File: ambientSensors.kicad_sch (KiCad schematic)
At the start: 14 parts, among them J2 BM04B-SRSS-TB, U1 LTR-329ALS-01, U3 TPS22914BYFPR, U7 BME688

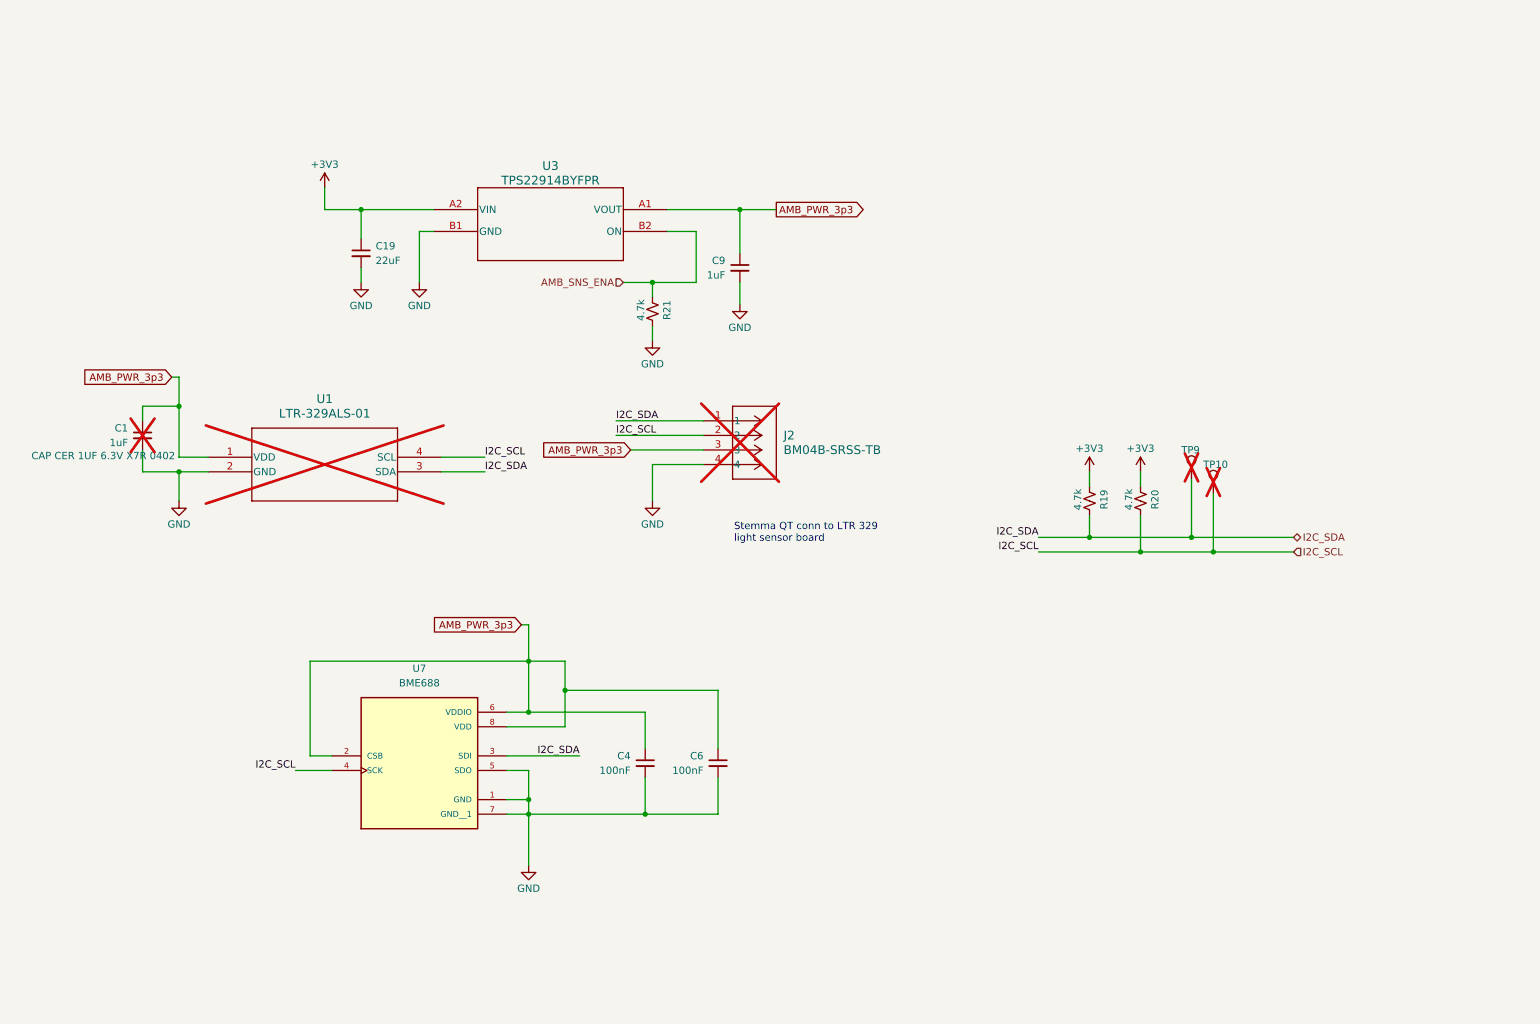
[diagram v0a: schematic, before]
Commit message: mutli soil sensor update
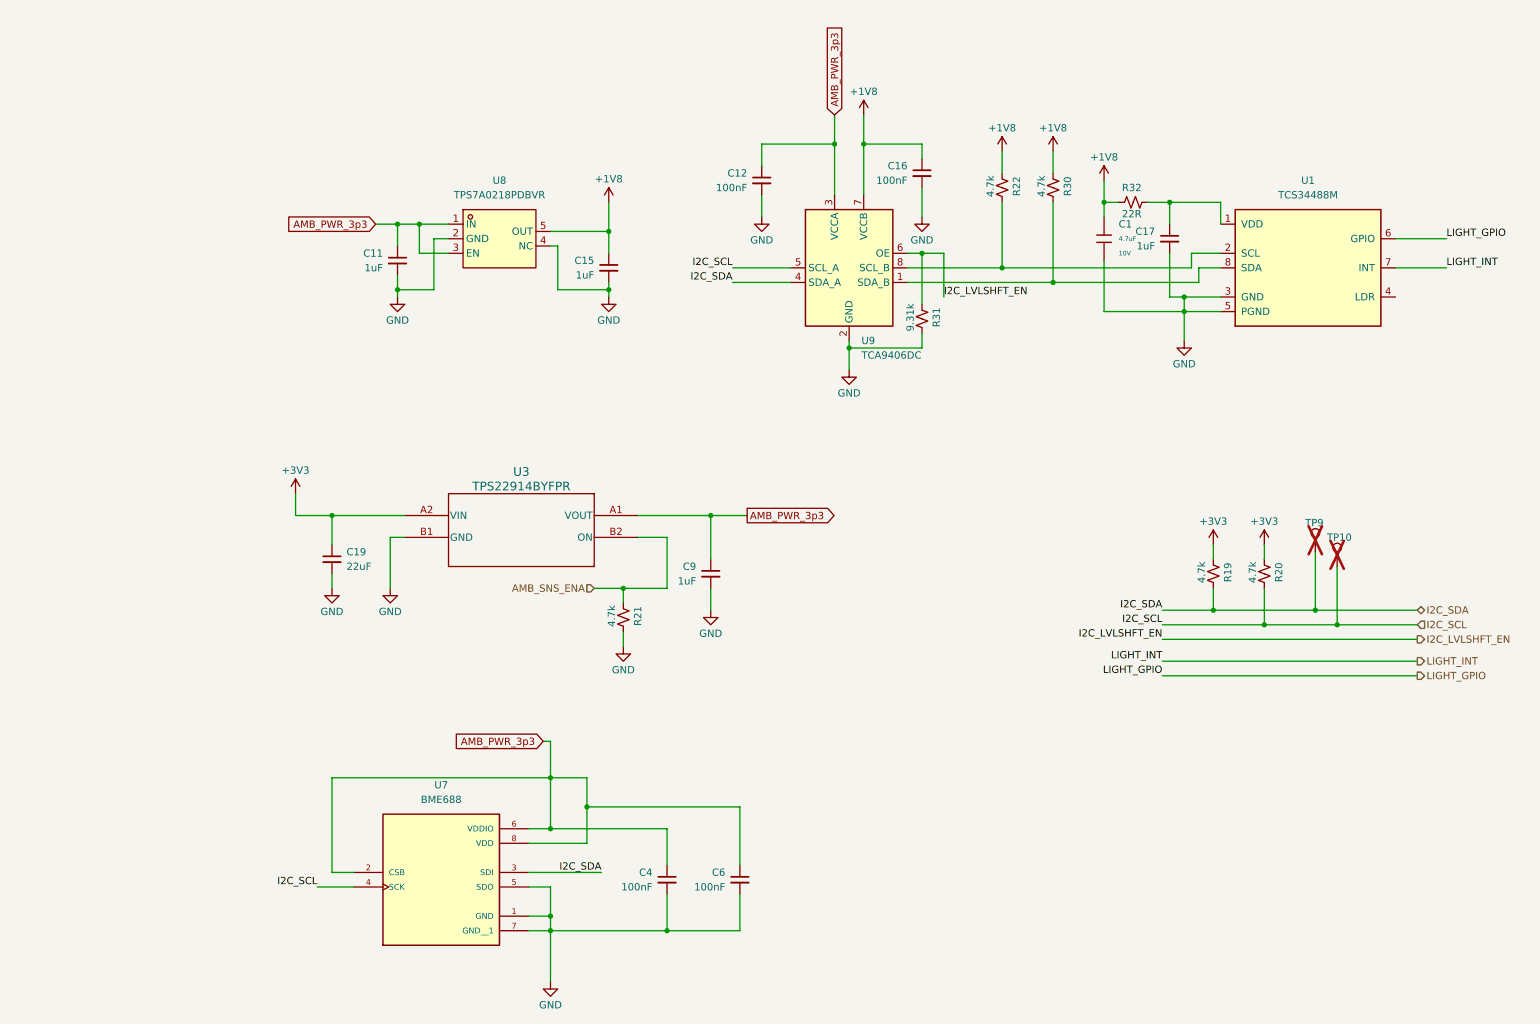
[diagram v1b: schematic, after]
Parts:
- removed C1: 1uF, Capacitor_SMD:C_0402_1005Metric, symbol Device:C_Small
- removed J2: BM04B-SRSS-TB, SproutSenseFootprints:CONN4_BM04B-SRSS_JST, symbol SproutSense:BM04B-SRSS-TB
- removed U1: LTR-329ALS-01, SproutSenseFootprints:LTR-329ALS-01_LTO, symbol SproutSense:LTR-329ALS-01
- added C1: 4.7uF, PCM_JLCPCB:C_0402, symbol PCM_JLCPCB-Capacitors:0402,4.7uF
- added C11, C15, C17: 1uF, Capacitor_SMD:C_0402_1005Metric, symbol Device:C_Small
- added C12, C16: 100nF, Capacitor_SMD:C_0402_1005Metric, symbol Device:C_Small
- added R22, R30: 4.7k, Resistor_SMD:R_0402_1005Metric, symbol Device:R_Small_US
- added R31: 9.31k, Resistor_SMD:R_0402_1005Metric, symbol Device:R_Small_US
- added R32: 22R, Resistor_SMD:R_0402_1005Metric, symbol Device:R_Small_US
- added U1: TCS34488M, SproutSenseFootprints:8-TFLGA, symbol SproutSense:TCS34488M
- added U8: TPS7A0218PDBVR, EasyEDA:SOT-23-5_L2.9-W1.6-P0.95-LS2.8-BL, symbol EasyEDA:TPS7A0218PDBVR
- added U9: TCA9406DC, EasyEDA:SOT-23-5_L2.9-W1.6-P0.95-LS2.8-BL, symbol Interface:TCA9406DC
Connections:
- net AMB_PWR_3p3: now also C11.1, C12.1, U8.1 (IN), U8.3 (EN), U9.3 (VCCA)
- net GND: now also C1.2, C11.2, C12.2, C15.2, C16.2, C17.2, R31.1, U1.3 (GND), U1.5 (PGND), U8.2 (GND), U8.4 (NC), U9.2 (GND)
- net I2C_SCL: now also U9.5 (SCL_A)
- net I2C_SDA: now also U9.4 (SDA_A)
- new net: C17.1, R32.1, U1.1 (VDD)
- new net: R30.1, U1.8 (SDA), U9.1 (SDA_B)
- new net: R22.1, U1.2 (SCL), U9.8 (SCL_B)
- new net +1V8: C1.1, C15.1, C16.1, R22.2, R30.2, R32.2, U8.5 (OUT), U9.7 (VCCB)
- new net I2C_LVLSHFT_EN: R31.2, U9.6 (OE)
- new net LIGHT_GPIO: U1.6 (GPIO)
- new net LIGHT_INT: U1.7 (INT)
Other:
- note removed: "Stemma QT conn to LTR 329 light sensor board"
- moved on the sheet: C19, C4, C6, C9, R19, R20, R21, TP10, TP9, U3, U7
